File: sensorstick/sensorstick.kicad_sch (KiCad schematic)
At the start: 5 parts, among them U1 ESP32-C3_SUPERMINI

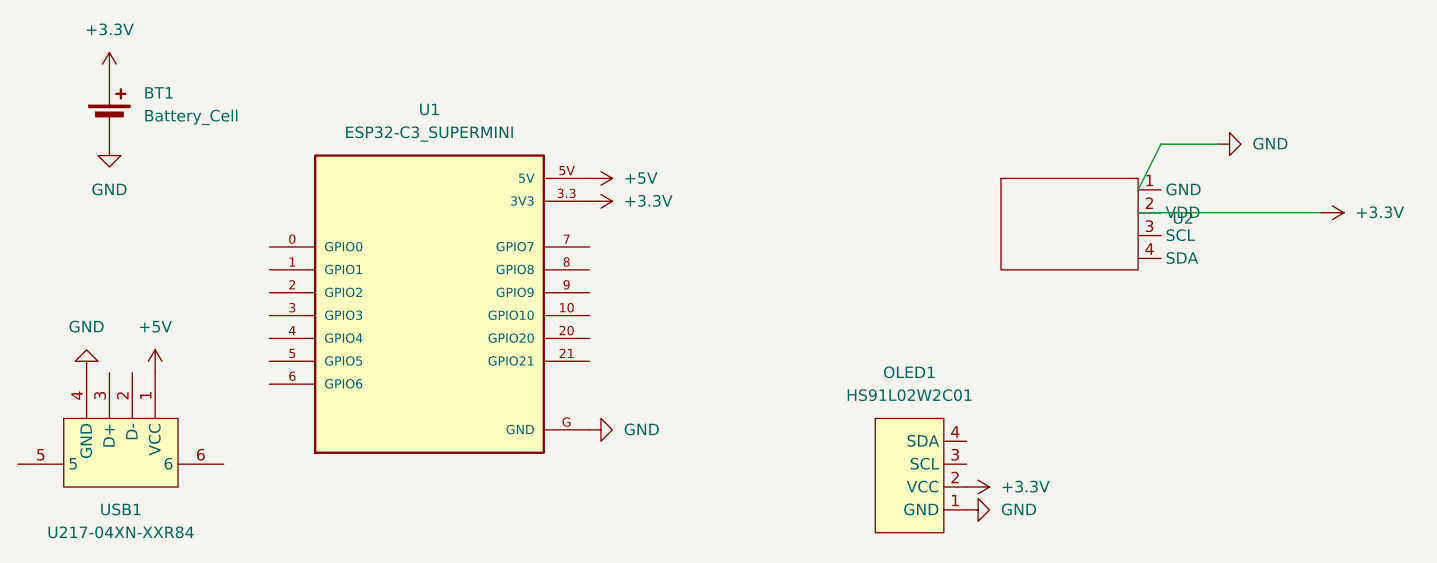
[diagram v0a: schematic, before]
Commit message: progress
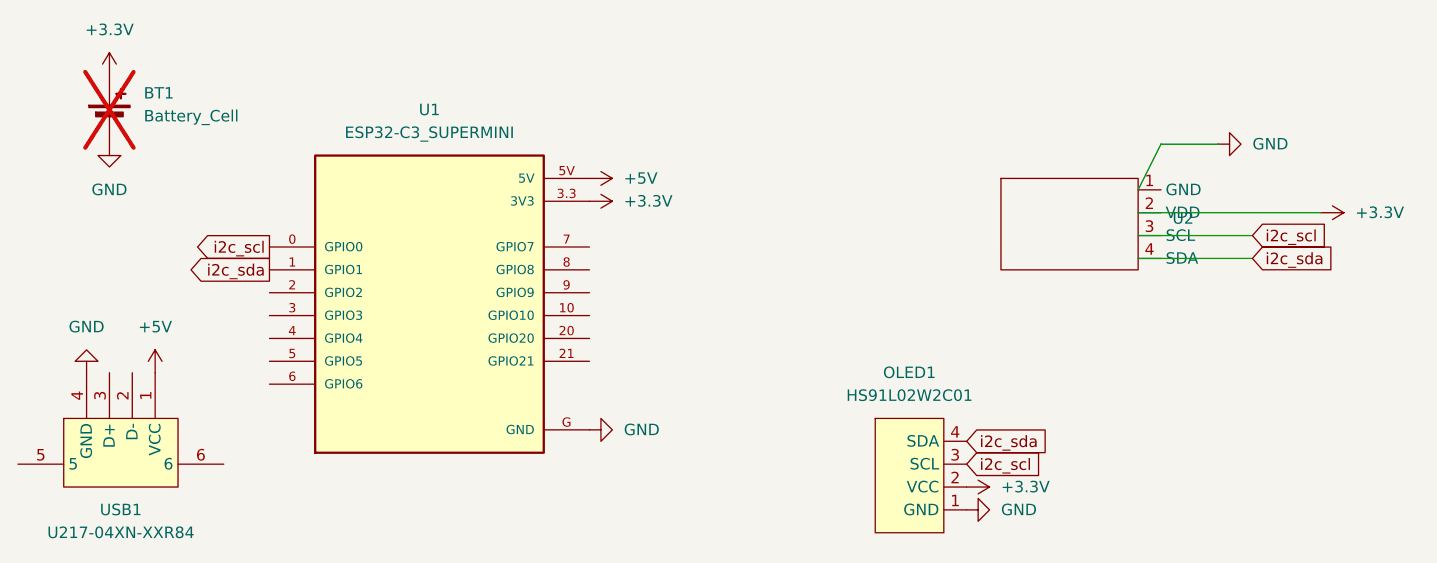
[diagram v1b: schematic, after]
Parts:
- BT1: now not fitted; now left out of the parts list
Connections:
- net i2c_scl: now reaches U1.0 (GPIO0)
- net i2c_scl: now also OLED1.3 (SCL), U2.3 (SCL)
- net i2c_sda: now reaches U1.1 (GPIO1)
- net i2c_sda: now also OLED1.4 (SDA), U2.4 (SDA)
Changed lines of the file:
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@@
+	(wire
+		(pts
+			(xy 142.24 46.99) (xy 154.94 46.99)
+		)
+		(stroke
+			(width 0)
+			(type default)
+		)
+	)
 	(wire
 		(pts
@@
 			(width 0)
 			(type default)
+		)
+	)
+	(wire
+		(pts
+			(xy 154.94 49.53) (xy 142.24 49.53)
+		)
+		(stroke
+			(width 0)
+			(type default)
+		)
+	)
+	(global_label "i2c_sda"
+		(shape input)
+		(at 154.94 49.53 0)
+		(fields_autoplaced yes)
+		(effects
+			(font
+				(size 1.27 1.27)
+			)
+			(justify left)
+		)
+		(property "Intersheetrefs" "${INTERSHEET_REFS}"
+			(at 165.1218 49.53 0)
+			(effects
+				(font
+					(size 1.27 1.27)
+				)
+				(justify left)
+				(hide yes)
+			)
+		)
+	)
+	(global_label "i2c_sda"
+		(shape output)
+		(at 45.72 50.8 180)
+		(fields_autoplaced yes)
+		(effects
+			(font
+				(size 1.27 1.27)
+			)
+			(justify right)
+		)
+		(property "Intersheetrefs" "${INTERSHEET_REFS}"
+			(at 35.5382 50.8 0)
+			(effects
+				(font
+					(size 1.27 1.27)
+				)
+				(justify right)
+				(hide yes)
+			)
+		)
+	)
+	(global_label "i2c_scl"
+		(shape output)
+		(at 45.72 48.26 180)
+		(fields_autoplaced yes)
+		(effects
+			(font
+				(size 1.27 1.27)
+			)
+			(justify right)
+		)
+		(property "Intersheetrefs" "${INTERSHEET_REFS}"
+			(at 36.0824 48.26 0)
+			(effects
+				(font
+					(size 1.27 1.27)
+				)
+				(justify right)
+				(hide yes)
+			)
+		)
+	)
+	(global_label "i2c_sda"
+		(shape input)
+		(at 123.19 69.85 0)
+		(fields_autoplaced yes)
+		(effects
+			(font
+				(size 1.27 1.27)
+			)
+			(justify left)
+		)
+		(property "Intersheetrefs" "${INTERSHEET_REFS}"
+			(at 133.3718 69.85 0)
+			(effects
+				(font
+					(size 1.27 1.27)
+				)
+				(justify left)
+				(hide yes)
+			)
+		)
+	)
+	(global_label "i2c_scl"
+		(shape input)
+		(at 123.19 72.39 0)
+		(fields_autoplaced yes)
+		(effects
+			(font
+				(size 1.27 1.27)
+			)
+			(justify left)
+		)
+		(property "Intersheetrefs" "${INTERSHEET_REFS}"
+			(at 132.8276 72.39 0)
+			(effects
+				(font
+					(size 1.27 1.27)
+				)
+				(justify left)
+				(hide yes)
+			)
+		)
+	)
+	(global_label "i2c_scl"
+		(shape input)
+		(at 154.94 46.99 0)
+		(fields_autoplaced yes)
+		(effects
+			(font
+				(size 1.27 1.27)
+			)
+			(justify left)
+		)
+		(property "Intersheetrefs" "${INTERSHEET_REFS}"
+			(at 164.5776 46.99 0)
+			(effects
+				(font
+					(size 1.27 1.27)
+				)
+				(justify left)
+				(hide yes)
+			)
 		)
 	)
@@
 		(at 27.94 34.29 0)
 		(unit 1)
-		(exclude_from_sim no)
-		(in_bom yes)
-		(on_board yes)
-		(dnp no)
+		(exclude_from_sim yes)
+		(in_bom no)
+		(on_board no)
+		(dnp yes)
 		(fields_autoplaced yes)
 		(property "Reference" "BT1"
